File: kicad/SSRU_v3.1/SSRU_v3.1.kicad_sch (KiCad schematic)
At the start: 91 parts, among them J1 Conn_01x03, J2 Conn_01x24, J3 Conn_02x03_Odd_Even, J31 Conn_01x04, J4 AVR-ISP-6, J5 Conn_01x03, SW1 SW_Push, U1 MCP2515-xSO, U10 TJA1051T, U11 TCA9517D, U12 TJA1051T, U13 CH340N, U2 ATmega328P-A, U3 LM2904, U4 LM2576S-5, U5 AMS1117-3.3, U7 MCP2515-xSO, U8 74LVC1G17, U9 MT3608/SDB628, Y1 16MHz, Y3 20MHz, Y4 20MHz

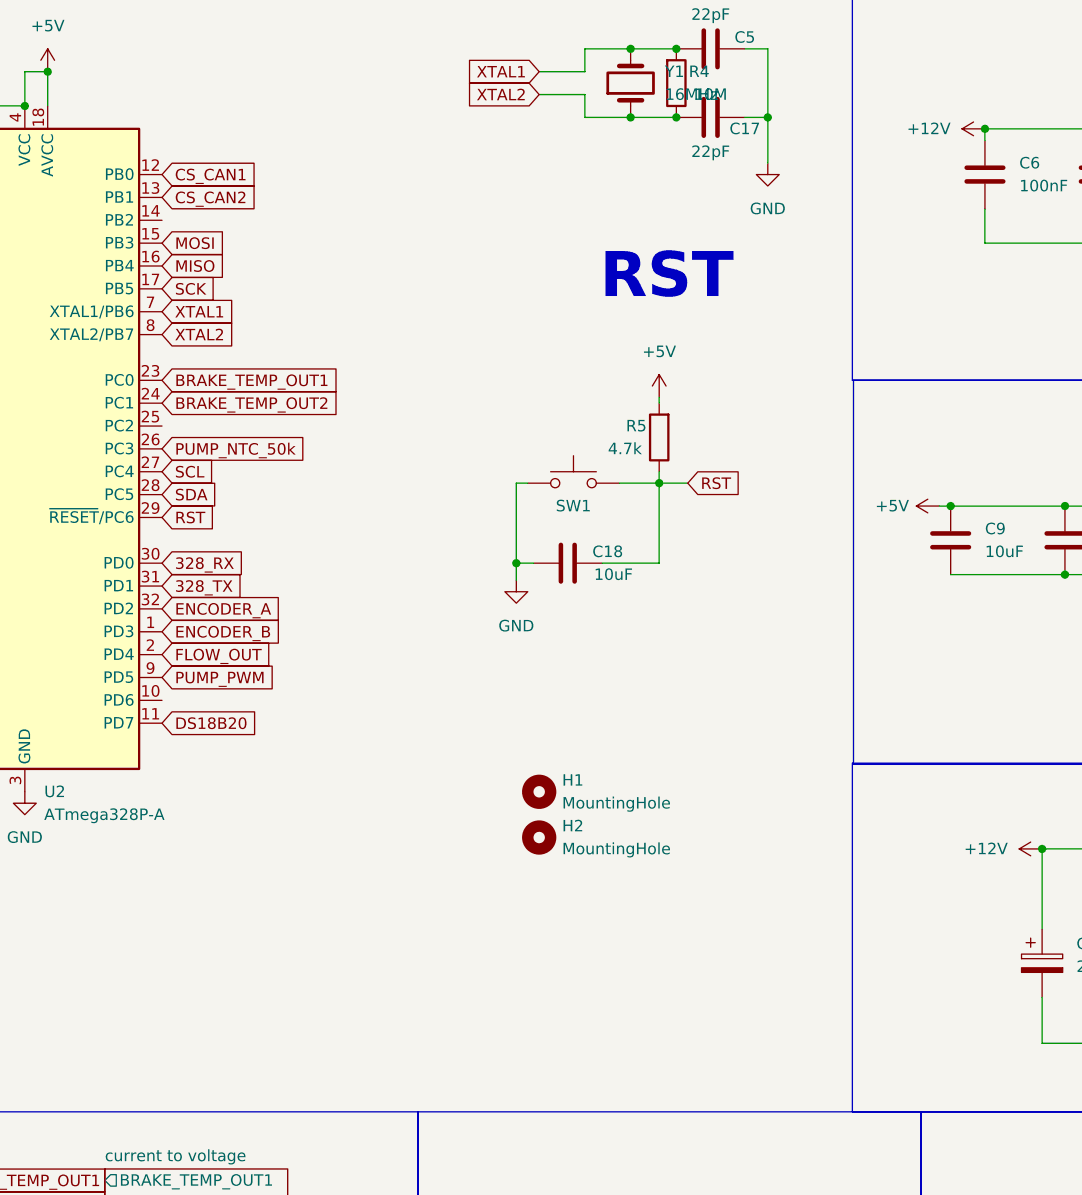
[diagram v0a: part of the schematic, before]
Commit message: SSRU
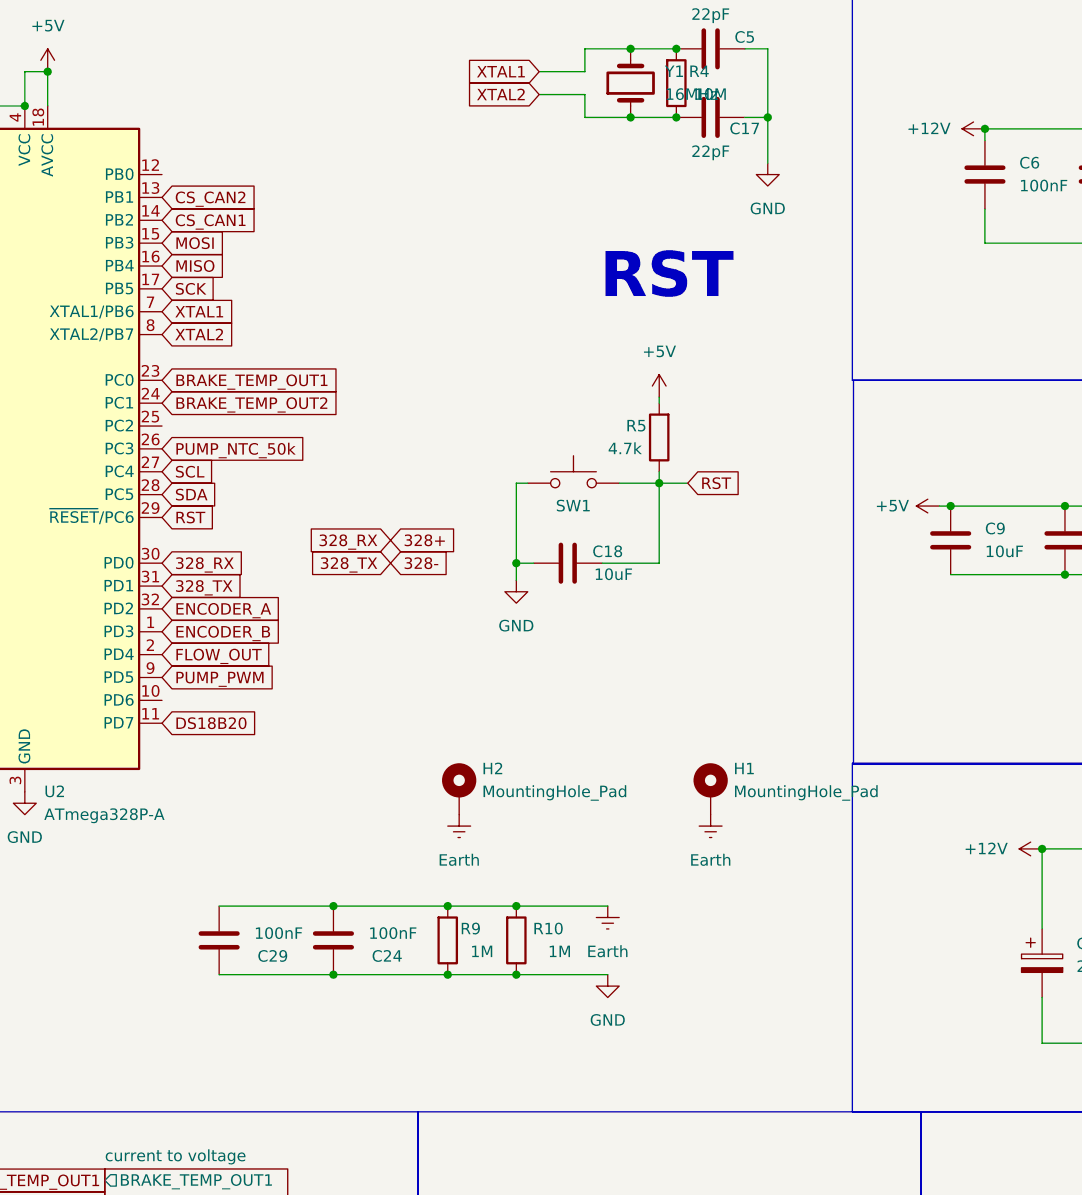
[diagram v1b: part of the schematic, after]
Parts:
- removed H1, H2: MountingHole, MountingHole:MountingHole_3.2mm_M3, symbol Mechanical:MountingHole
- added C24, C29: 100nF, RMC_Capacitor:C_0805_2012Metric_Pad1.18x1.45mm_HandSolder_L, symbol Device:C
- added H1, H2: MountingHole_Pad, MountingHole:MountingHole_3.2mm_M3_ISO14580_Pad, symbol Mechanical:MountingHole_Pad
- added R10, R9: 1M, RMC_Resistor:R_0805_2012Metric_Pad1.20x1.40mm_HandSolder_L, symbol Device:R
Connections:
- net CS_CAN1: now also U2.14 (PB2); no longer U2.12 (PB0)
- net GND: now also C24.1, C29.1, R10.1, R9.1
- net 328_RX renamed 328+
- net 328_TX renamed 328-
- new net Earth: C24.2, C29.2, H1.1, H2.1, R10.2, R9.2

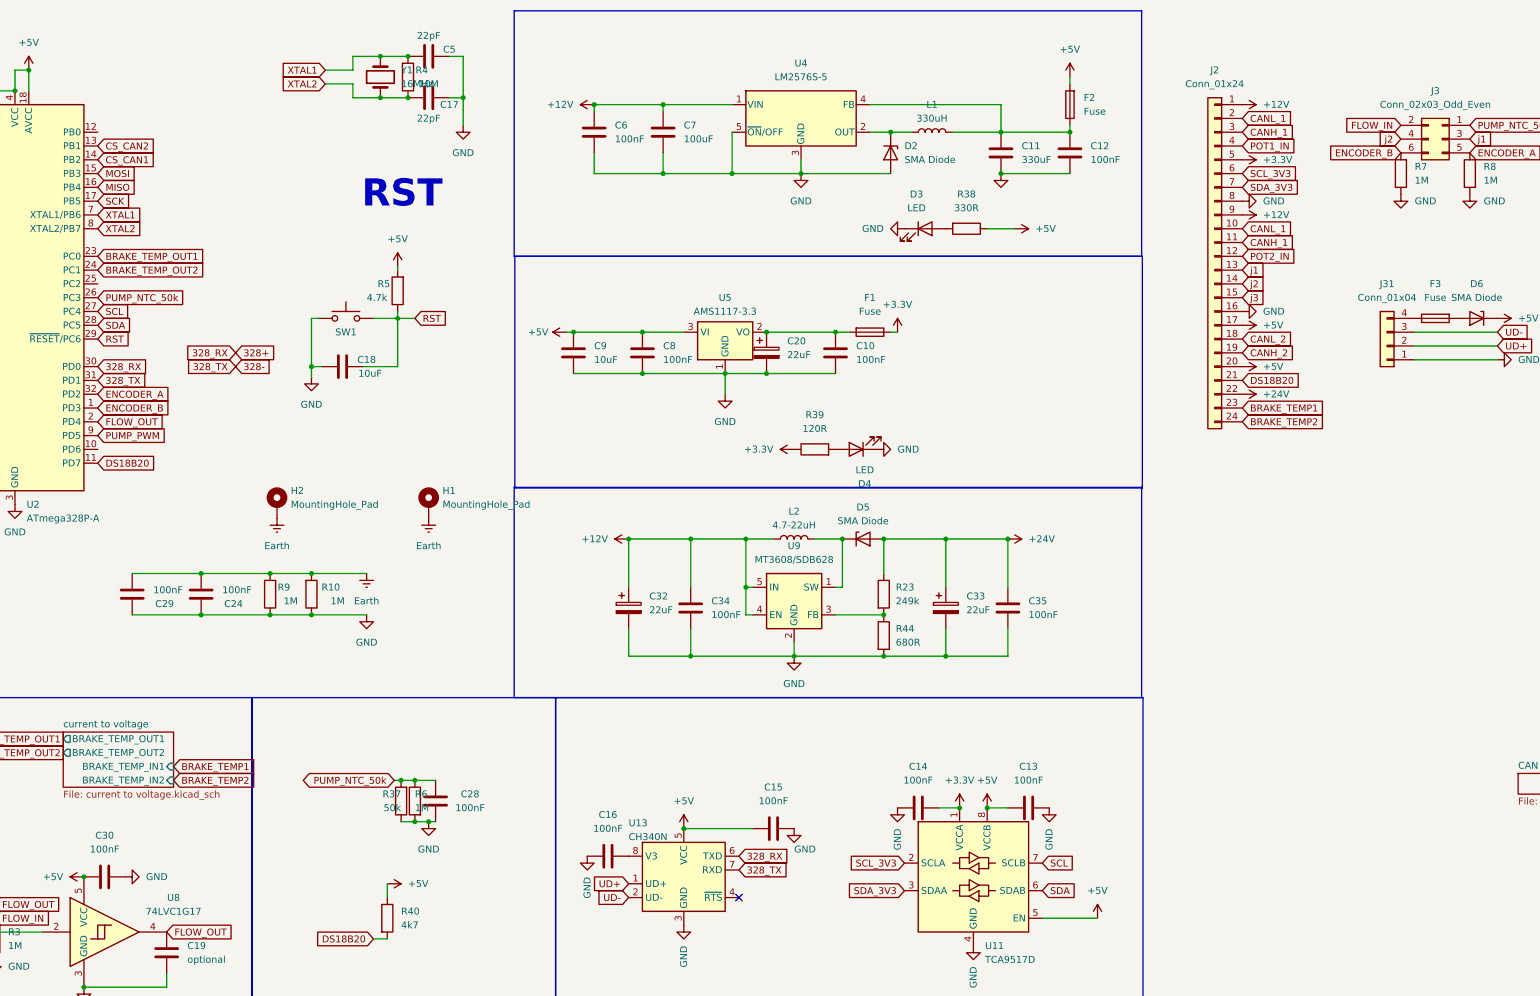
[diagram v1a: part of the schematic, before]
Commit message: sorry I loved you
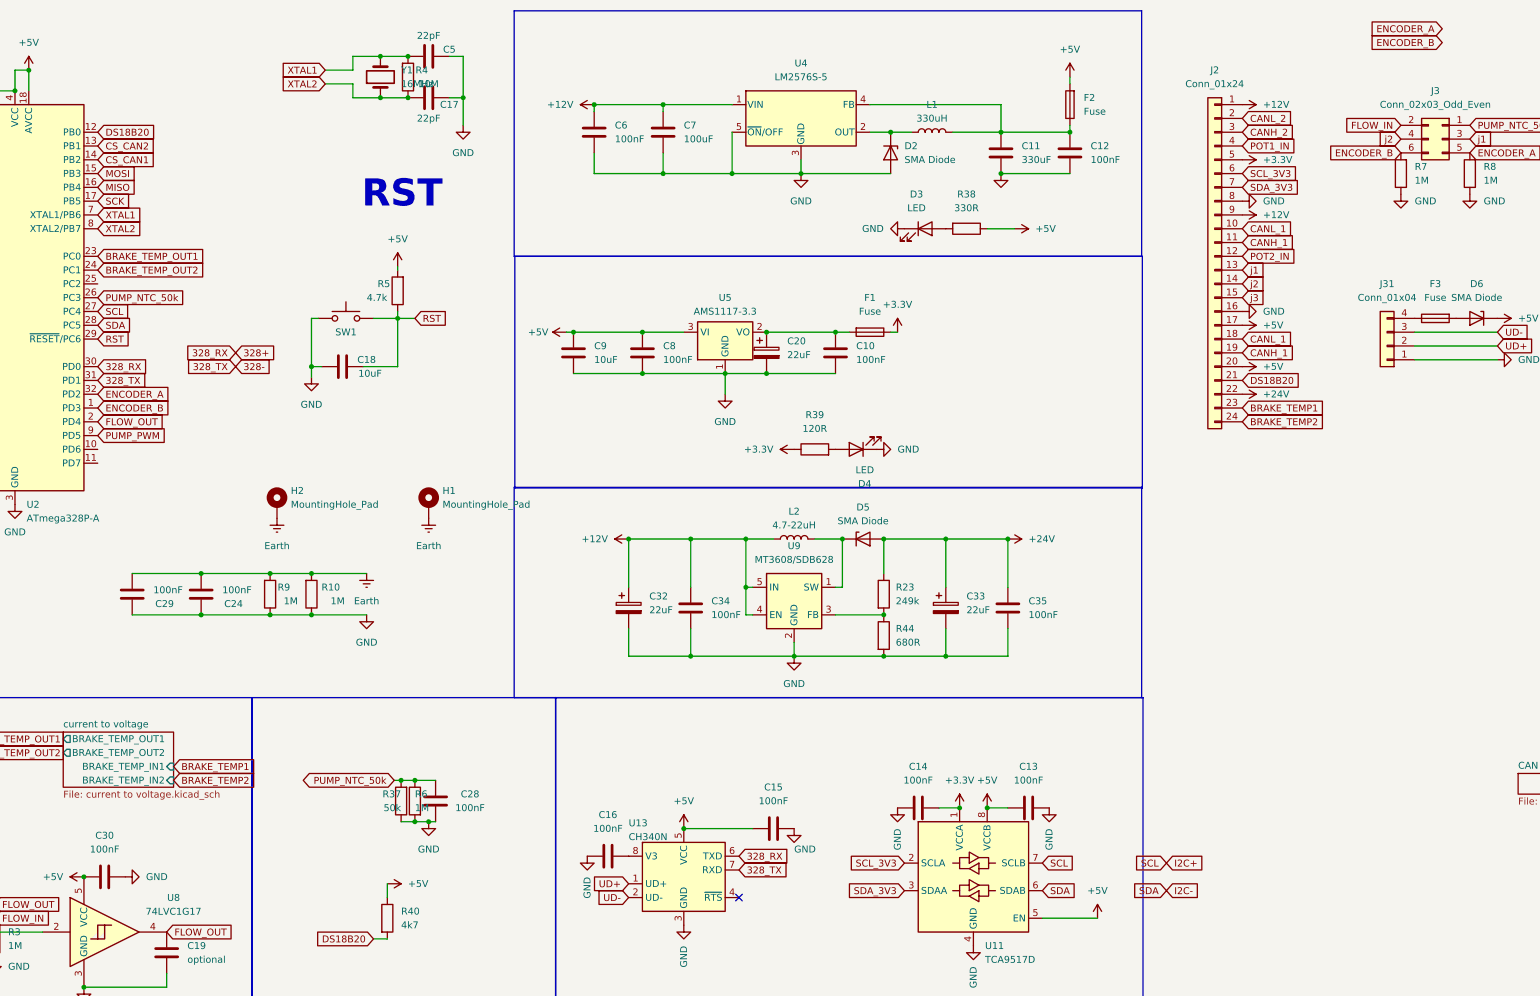
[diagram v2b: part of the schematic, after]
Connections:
- net CAN1+: now also J2.19 (Pin_19); no longer J2.3 (Pin_3)
- net CAN1-: now also J2.18 (Pin_18); no longer J2.2 (Pin_2)
- net CAN2+: now also J2.3 (Pin_3); no longer J2.19 (Pin_19)
- net CAN2-: now also J2.2 (Pin_2); no longer J2.18 (Pin_18)
- net DS18B20: now also U2.12 (PB0); no longer U2.11 (PD7)
- net SCL renamed I2C+
- net SDA renamed I2C-

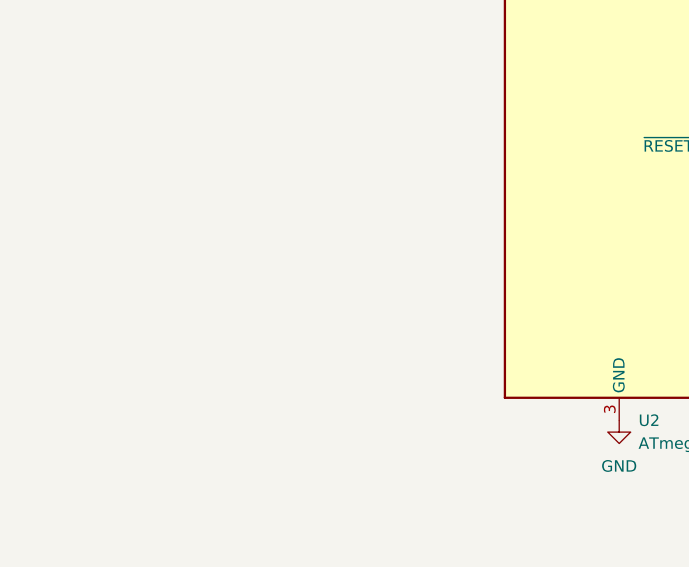
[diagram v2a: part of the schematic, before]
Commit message: gerbers
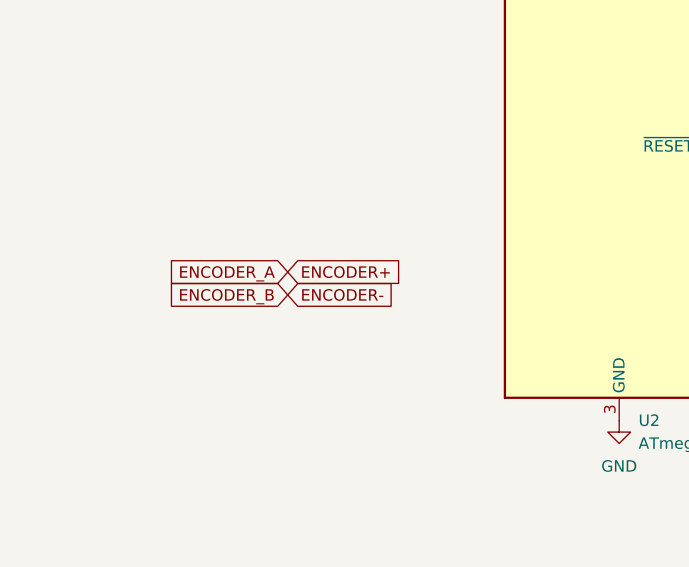
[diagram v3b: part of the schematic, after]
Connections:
- net ENCODER_A renamed ENCODER+
- net ENCODER_B renamed ENCODER-
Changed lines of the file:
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@@
+		)
+	)
+	(global_label "ENCODER-"
+		(shape input)
+		(at 40.64 88.9 0)
+		(fields_autoplaced yes)
+		(effects
+			(font
+				(size 1.27 1.27)
+			)
+			(justify left)
+		)
+		(property "Intersheetrefs" "${INTERSHEET_REFS}"
+			(at 53.9666 88.9 0)
+			(effects
+				(font
+					(size 1.27 1.27)
+				)
+				(justify left)
+				(hide yes)
+			)
 		)
 	)
@@
 		)
 	)
+	(global_label "ENCODER_A"
+		(shape input)
+		(at 40.64 86.36 180)
+		(fields_autoplaced yes)
+		(effects
+			(font
+				(size 1.27 1.27)
+			)
+			(justify right)
+		)
+		(property "Intersheetrefs" "${INTERSHEET_REFS}"
+			(at 26.8296 86.36 0)
+			(effects
+				(font
+					(size 1.27 1.27)
+				)
+				(justify right)
+				(hide yes)
+			)
+		)
+	)
 	(global_label "ENCODER_B"
 		(shape input)
@@
 		)
 	)
+	(global_label "ENCODER_B"
+		(shape input)
+		(at 40.64 88.9 180)
+		(fields_autoplaced yes)
+		(effects
+			(font
+				(size 1.27 1.27)
+			)
+			(justify right)
+		)
+		(property "Intersheetrefs" "${INTERSHEET_REFS}"
+			(at 26.6482 88.9 0)
+			(effects
+				(font
+					(size 1.27 1.27)
+				)
+				(justify right)
+				(hide yes)
+			)
+		)
+	)
 	(global_label "CANH_2"
 		(shape input)
@@
 			(effects
 				(font
+					(size 1.27 1.27)
+				)
+				(justify left)
+				(hide yes)
+			)
+		)
+	)
+	(global_label "ENCODER+"
+		(shape input)
+		(at 40.64 86.36 0)
+		(fields_autoplaced yes)
+		(effects
+			(font
+				(size 1.27 1.27)
+			)
+			(justify left)
+		)
+		(property "Intersheetrefs" "${INTERSHEET_REFS}"
+			(at 53.9666 86.36 0)
+			(effects
+				(font
